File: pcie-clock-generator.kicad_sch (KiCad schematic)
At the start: 7 parts, among them U31 SI52112-B6-GT, Y6 Resonator_25MHz_ABM8G

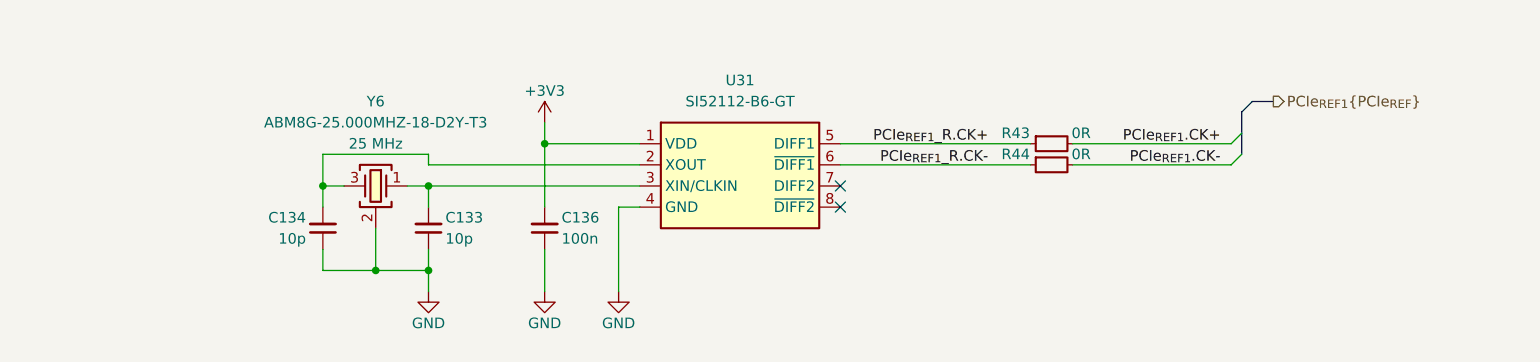
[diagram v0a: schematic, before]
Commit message: [#79790] Applied review fixes
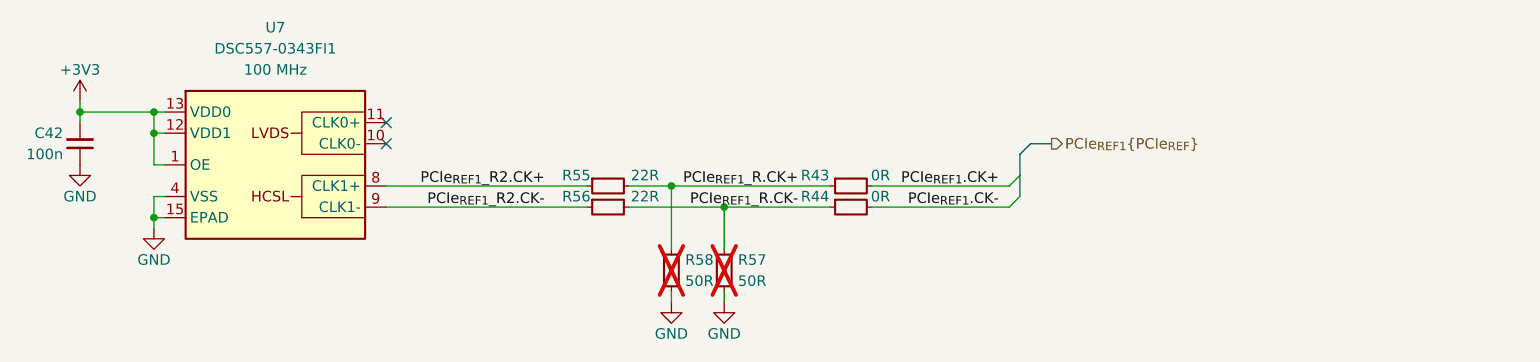
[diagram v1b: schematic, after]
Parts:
- removed C133, C134: C_10p_25V_0402, antmicro-footprints:C_0402_1005Metric, symbol antmicroCapacitors0402:C_10p_25V_0402
- removed C136: C_100n_0402, antmicro-footprints:C_0402_1005Metric, symbol antmicroCapacitors0402:C_100n_0402
- removed U31: SI52112-B6-GT, antmicro-footprints:TSSOP-8_3x4.4mm_P0.65mm, symbol antmicroClockTimingClockGeneratorsPLLsFrequencySynthesizers:SI52112-B6-GT
- removed Y6: Resonator_25MHz_ABM8G, antmicro-footprints:Resonator_SMD_Abracon_ABM8G_3.2x2.5mm, symbol antmicroResonators:Resonator_25MHz_ABM8G
- added C42: C_100n_0402, antmicro-footprints:C_0402_1005Metric, symbol antmicroCapacitors0402:C_100n_0402
- added R55, R56: R_22R_0402, antmicro-footprints:R_0402_1005Metric, symbol antmicroResistors0402:R_22R_0402
- added R57, R58: R_50R_0402, antmicro-footprints:R_0402_1005Metric, symbol antmicroResistors0402:R_50R_0402
- added U7: DSC557-0343FI1, antmicro-footprints:VQFN-14-1EP_3.2x2.5mm_P0.5mm_Layout4x3, symbol antmicroClockTimingRealTimeClocks:DSC557-0343FI1
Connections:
- net +3V3: now also C42.2, U7.1 (OE), U7.12 (VDD1), U7.13 (VDD0)
- net GND: now also C42.1, R57.1, R58.1, U7.15 (EPAD), U7.4 (VSS)
- net PCIe_{REF1}_R.CK+: now also R55.2, R58.2
- net PCIe_{REF1}_R.CK-: now also R56.2, R57.2
- new net PCIe_{REF1}_R2.CK+: R55.1, U7.8 (CLK1+)
- new net PCIe_{REF1}_R2.CK-: R56.1, U7.9 (CLK1-)
